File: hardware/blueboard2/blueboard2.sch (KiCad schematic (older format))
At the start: 142 parts, among them Q1 TRANSISTOR_NPN, Q2 TRANSISTOR_NPN, Q3 TRANSISTOR_NPN, SW2 SW_PUSHBUTTON

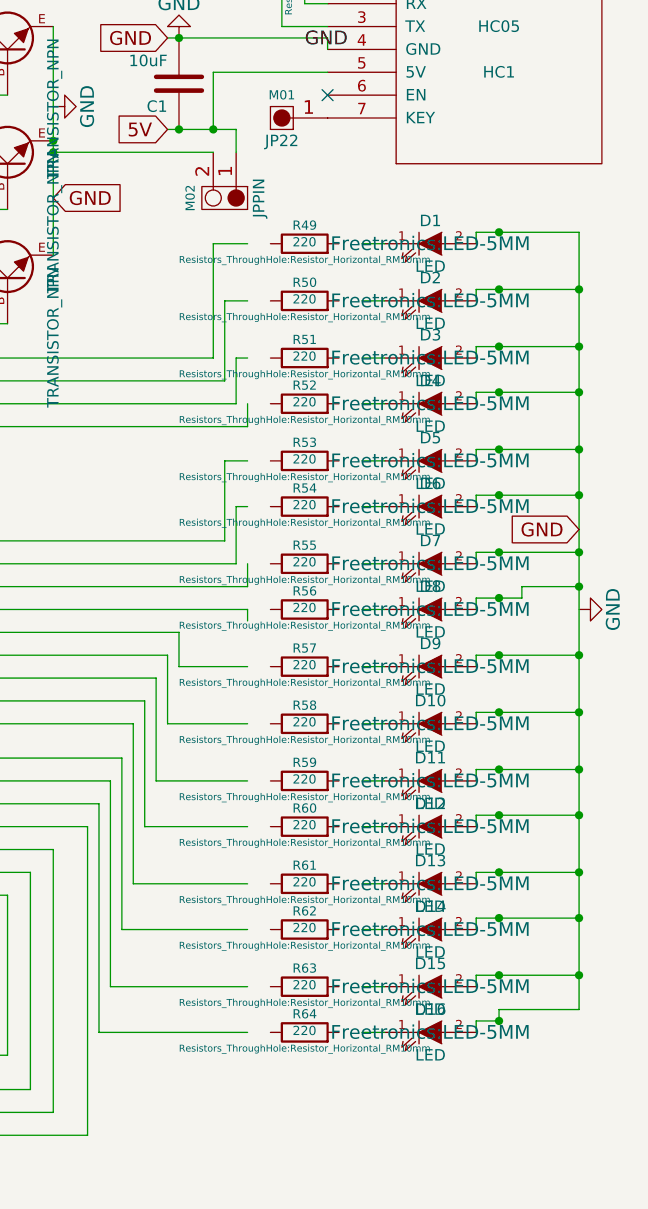
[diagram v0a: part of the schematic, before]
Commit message: lots of changes
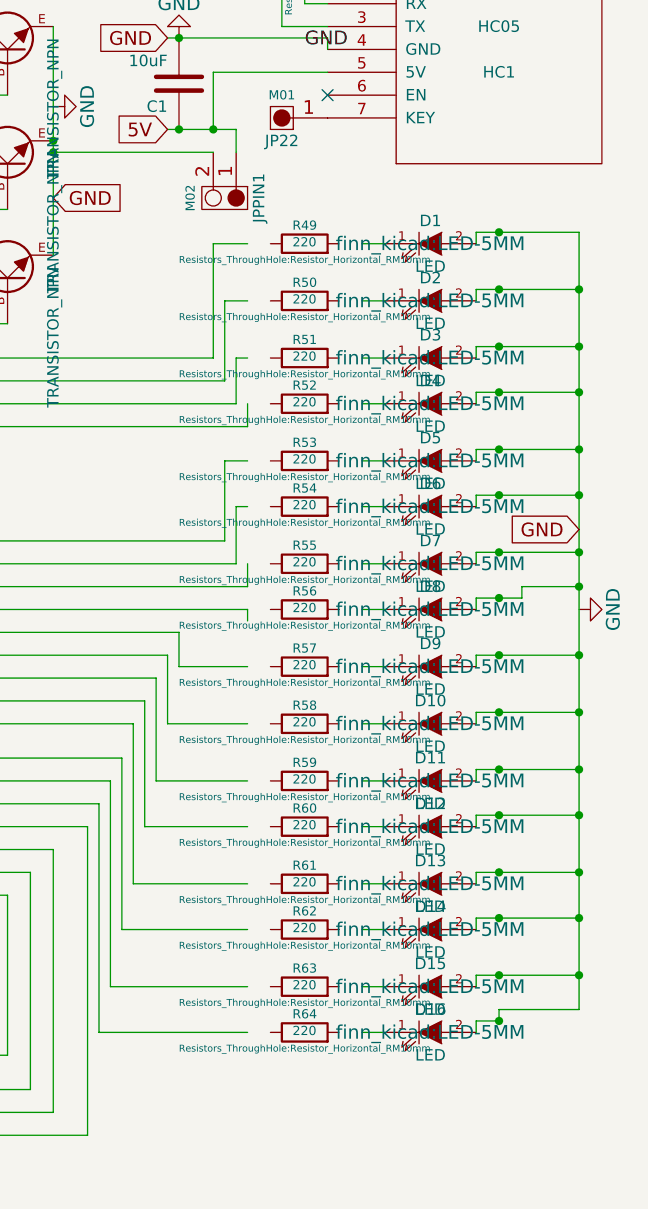
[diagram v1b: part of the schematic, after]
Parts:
- D1, D10, D11, D12, D13, D14, D15, D16, D2, D3, D4, D5, D6, D7, D8, D9: footprint Freetronics:LED-5MM -> finn_kicad:LED-5MM
- JPPIN1: renamed from JPPIN; footprint (none) -> Freetronics:1X02
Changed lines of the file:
@@
 F 0 "D3" H 10450 4200 50  0000 C CNN
 F 1 "LED" H 10450 4000 50  0000 C CNN
-F 2 "Freetronics:LED-5MM" H 10450 4100 60  0000 C CNN
+F 2 "finn_kicad:LED-5MM" H 10450 4100 60  0000 C CNN
 F 3 "~" H 10450 4100 60  0000 C CNN
 	1    10450 4100
@@
 F 0 "D2" H 10450 3950 50  0000 C CNN
 F 1 "LED" H 10450 3750 50  0000 C CNN
-F 2 "Freetronics:LED-5MM" H 10450 3850 60  0000 C CNN
+F 2 "finn_kicad:LED-5MM" H 10450 3850 60  0000 C CNN
 F 3 "~" H 10450 3850 60  0000 C CNN
 	1    10450 3850
@@
 F 0 "D5" H 10450 4650 50  0000 C CNN
 F 1 "LED" H 10450 4450 50  0000 C CNN
-F 2 "Freetronics:LED-5MM" H 10450 4550 60  0000 C CNN
+F 2 "finn_kicad:LED-5MM" H 10450 4550 60  0000 C CNN
 F 3 "~" H 10450 4550 60  0000 C CNN
 	1    10450 4550
@@
 F 0 "D4" H 10450 4400 50  0000 C CNN
 F 1 "LED" H 10450 4200 50  0000 C CNN
-F 2 "Freetronics:LED-5MM" H 10450 4300 60  0000 C CNN
+F 2 "finn_kicad:LED-5MM" H 10450 4300 60  0000 C CNN
 F 3 "~" H 10450 4300 60  0000 C CNN
 	1    10450 4300
@@
 F 0 "D7" H 10450 5100 50  0000 C CNN
 F 1 "LED" H 10450 4900 50  0000 C CNN
-F 2 "Freetronics:LED-5MM" H 10450 5000 60  0000 C CNN
+F 2 "finn_kicad:LED-5MM" H 10450 5000 60  0000 C CNN
 F 3 "~" H 10450 5000 60  0000 C CNN
 	1    10450 5000
@@
 F 0 "D6" H 10450 4850 50  0000 C CNN
 F 1 "LED" H 10450 4650 50  0000 C CNN
-F 2 "Freetronics:LED-5MM" H 10450 4750 60  0000 C CNN
+F 2 "finn_kicad:LED-5MM" H 10450 4750 60  0000 C CNN
 F 3 "~" H 10450 4750 60  0000 C CNN
 	1    10450 4750
@@
 F 0 "D9" H 10450 5550 50  0000 C CNN
 F 1 "LED" H 10450 5350 50  0000 C CNN
-F 2 "Freetronics:LED-5MM" H 10450 5450 60  0000 C CNN
+F 2 "finn_kicad:LED-5MM" H 10450 5450 60  0000 C CNN
 F 3 "~" H 10450 5450 60  0000 C CNN
 	1    10450 5450
@@
 F 0 "D8" H 10450 5300 50  0000 C CNN
 F 1 "LED" H 10450 5100 50  0000 C CNN
-F 2 "Freetronics:LED-5MM" H 10450 5200 60  0000 C CNN
+F 2 "finn_kicad:LED-5MM" H 10450 5200 60  0000 C CNN
 F 3 "~" H 10450 5200 60  0000 C CNN
 	1    10450 5200
@@
 F 0 "D11" H 10450 6050 50  0000 C CNN
 F 1 "LED" H 10450 5850 50  0000 C CNN
-F 2 "Freetronics:LED-5MM" H 10450 5950 60  0000 C CNN
+F 2 "finn_kicad:LED-5MM" H 10450 5950 60  0000 C CNN
 F 3 "~" H 10450 5950 60  0000 C CNN
 	1    10450 5950
@@
 F 0 "D10" H 10450 5800 50  0000 C CNN
 F 1 "LED" H 10450 5600 50  0000 C CNN
-F 2 "Freetronics:LED-5MM" H 10450 5700 60  0000 C CNN
+F 2 "finn_kicad:LED-5MM" H 10450 5700 60  0000 C CNN
 F 3 "~" H 10450 5700 60  0000 C CNN
 	1    10450 5700
@@
 F 0 "D13" H 10450 6500 50  0000 C CNN
 F 1 "LED" H 10450 6300 50  0000 C CNN
-F 2 "Freetronics:LED-5MM" H 10450 6400 60  0000 C CNN
+F 2 "finn_kicad:LED-5MM" H 10450 6400 60  0000 C CNN
 F 3 "~" H 10450 6400 60  0000 C CNN
 	1    10450 6400
@@
 F 0 "D12" H 10450 6250 50  0000 C CNN
 F 1 "LED" H 10450 6050 50  0000 C CNN
-F 2 "Freetronics:LED-5MM" H 10450 6150 60  0000 C CNN
+F 2 "finn_kicad:LED-5MM" H 10450 6150 60  0000 C CNN
 F 3 "~" H 10450 6150 60  0000 C CNN
 	1    10450 6150
@@
 F 0 "D15" H 10450 6950 50  0000 C CNN
 F 1 "LED" H 10450 6750 50  0000 C CNN
-F 2 "Freetronics:LED-5MM" H 10450 6850 60  0000 C CNN
+F 2 "finn_kicad:LED-5MM" H 10450 6850 60  0000 C CNN
 F 3 "~" H 10450 6850 60  0000 C CNN
 	1    10450 6850
@@
 F 0 "D14" H 10450 6700 50  0000 C CNN
 F 1 "LED" H 10450 6500 50  0000 C CNN
-F 2 "Freetronics:LED-5MM" H 10450 6600 60  0000 C CNN
+F 2 "finn_kicad:LED-5MM" H 10450 6600 60  0000 C CNN
 F 3 "~" H 10450 6600 60  0000 C CNN
 	1    10450 6600
@@
 F 0 "D1" H 10450 3700 50  0000 C CNN
 F 1 "LED" H 10450 3500 50  0000 C CNN
-F 2 "Freetronics:LED-5MM" H 10450 3600 60  0000 C CNN
+F 2 "finn_kicad:LED-5MM" H 10450 3600 60  0000 C CNN
 F 3 "~" H 10450 3600 60  0000 C CNN
 	1    10450 3600
@@
 F 0 "D16" H 10450 7150 50  0000 C CNN
 F 1 "LED" H 10450 6950 50  0000 C CNN
-F 2 "Freetronics:LED-5MM" H 10450 7050 60  0000 C CNN
+F 2 "finn_kicad:LED-5MM" H 10450 7050 60  0000 C CNN
 F 3 "~" H 10450 7050 60  0000 C CNN
 	1    10450 7050
@@
 $EndComp
 $Comp
-L M02 JPPIN
+L M02 JPPIN1
 U 1 1 550D02A5
 P 9600 3500
-F 0 "JPPIN" H 9500 3600 50  0000 C CNN
+F 0 "JPPIN1" H 9500 3600 50  0000 C CNN
 F 1 "M02" H 9500 3300 40  0000 C CNN
-F 2 "" H 9600 3500 60  0000 C CNN
+F 2 "Freetronics:1X02" H 9600 3500 60  0001 C CNN
 F 3 "" H 9600 3500 60  0000 C CNN
 	1    9600 3500
